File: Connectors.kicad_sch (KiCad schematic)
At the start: 4 parts

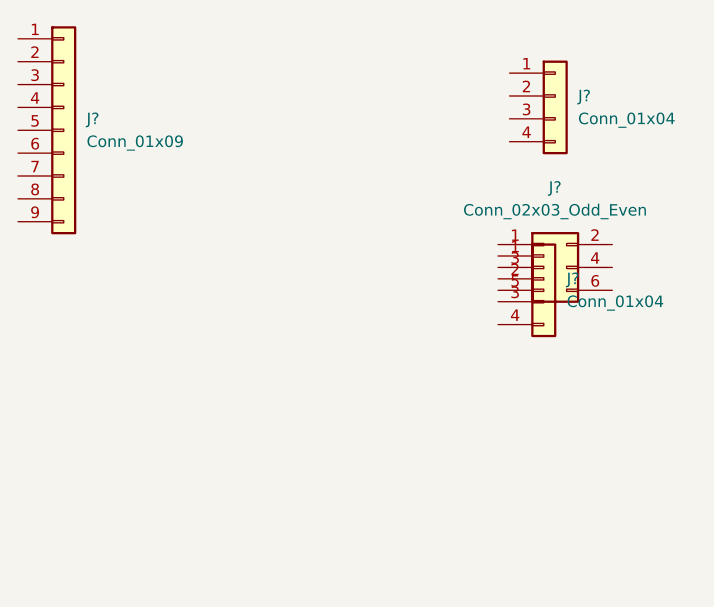
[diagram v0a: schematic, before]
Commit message: Annotation
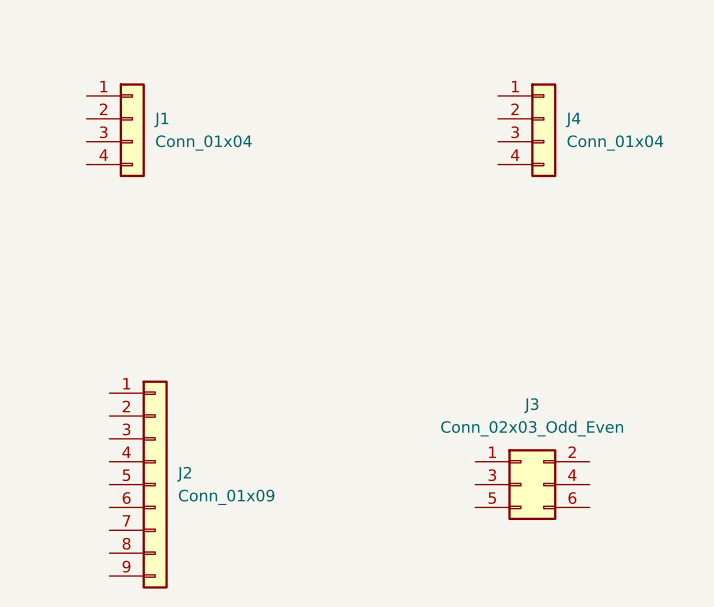
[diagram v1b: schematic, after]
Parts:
- gave numbers to parts that had none: 4
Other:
- moved on the sheet: J1, J2, J3, J4
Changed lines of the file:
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@@
     (company "GM Industries")
   )
-  (symbol (lib_id "Connector_Generic:Conn_01x09") (at 91.44 59.69 0) (unit 1)
+  (symbol (lib_id "Connector_Generic:Conn_01x09") (at 101.6 99.06 0) (unit 1)
     (in_bom yes) (on_board yes) (fields_autoplaced)
-    (property "Reference" "J?" (id 0) (at 93.98 58.4199 0)
+    (property "Reference" "J2" (id 0) (at 104.14 97.7899 0)
       (effects (font (size 1.27 1.27)) (justify left))
     )
-    (property "Value" "Conn_01x09" (id 1) (at 93.98 60.9599 0)
+    (property "Value" "Conn_01x09" (id 1) (at 104.14 100.3299 0)
       (effects (font (size 1.27 1.27)) (justify left))
     )
-    (property "Footprint" "" (id 2) (at 91.44 59.69 0)
+    (property "Footprint" "" (id 2) (at 101.6 99.06 0)
       (effects (font (size 1.27 1.27)) hide)
     )
-    (property "Datasheet" "~" (id 3) (at 91.44 59.69 0)
+    (property "Datasheet" "~" (id 3) (at 101.6 99.06 0)
       (effects (font (size 1.27 1.27)) hide)
     )
@@
     (pin "9")
   )
-  (symbol (lib_id "Connector_Generic:Conn_02x03_Odd_Even") (at 144.78 74.93 0) (unit 1)
+  (symbol (lib_id "Connector_Generic:Conn_02x03_Odd_Even") (at 142.24 99.06 0) (unit 1)
     (in_bom yes) (on_board yes) (fields_autoplaced)
-    (property "Reference" "J?" (id 0) (at 146.05 66.04 0))
-    (property "Value" "Conn_02x03_Odd_Even" (id 1) (at 146.05 68.58 0))
-    (property "Footprint" "" (id 2) (at 144.78 74.93 0)
+    (property "Reference" "J3" (id 0) (at 143.51 90.17 0))
+    (property "Value" "Conn_02x03_Odd_Even" (id 1) (at 143.51 92.71 0))
+    (property "Footprint" "" (id 2) (at 142.24 99.06 0)
       (effects (font (size 1.27 1.27)) hide)
     )
-    (property "Datasheet" "~" (id 3) (at 144.78 74.93 0)
+    (property "Datasheet" "~" (id 3) (at 142.24 99.06 0)
       (effects (font (size 1.27 1.27)) hide)
     )
@@
     (pin "6")
   )
-  (symbol (lib_id "Connector_Generic:Conn_01x04") (at 144.78 76.2 0) (unit 1)
+  (symbol (lib_id "Connector_Generic:Conn_01x04") (at 144.78 58.42 0) (unit 1)
     (in_bom yes) (on_board yes) (fields_autoplaced)
-    (property "Reference" "J?" (id 0) (at 147.32 76.1999 0)
+    (property "Reference" "J4" (id 0) (at 147.32 58.4199 0)
       (effects (font (size 1.27 1.27)) (justify left))
     )
-    (property "Value" "Conn_01x04" (id 1) (at 147.32 78.7399 0)
+    (property "Value" "Conn_01x04" (id 1) (at 147.32 60.9599 0)
       (effects (font (size 1.27 1.27)) (justify left))
     )
-    (property "Footprint" "" (id 2) (at 144.78 76.2 0)
+    (property "Footprint" "" (id 2) (at 144.78 58.42 0)
       (effects (font (size 1.27 1.27)) hide)
     )
-    (property "Datasheet" "~" (id 3) (at 144.78 76.2 0)
+    (property "Datasheet" "~" (id 3) (at 144.78 58.42 0)
       (effects (font (size 1.27 1.27)) hide)
     )
@@
     (pin "4")
   )
-  (symbol (lib_id "Connector_Generic:Conn_01x04") (at 146.05 55.88 0) (unit 1)
+  (symbol (lib_id "Connector_Generic:Conn_01x04") (at 99.06 58.42 0) (unit 1)
     (in_bom yes) (on_board yes) (fields_autoplaced)
-    (property "Reference" "J?" (id 0) (at 148.59 55.8799 0)
+    (property "Reference" "J1" (id 0) (at 101.6 58.4199 0)
       (effects (font (size 1.27 1.27)) (justify left))
     )
-    (property "Value" "Conn_01x04" (id 1) (at 148.59 58.4199 0)
+    (property "Value" "Conn_01x04" (id 1) (at 101.6 60.9599 0)
       (effects (font (size 1.27 1.27)) (justify left))
     )
-    (property "Footprint" "" (id 2) (at 146.05 55.88 0)
+    (property "Footprint" "" (id 2) (at 99.06 58.42 0)
       (effects (font (size 1.27 1.27)) hide)
     )
-    (property "Datasheet" "~" (id 3) (at 146.05 55.88 0)
+    (property "Datasheet" "~" (id 3) (at 99.06 58.42 0)
       (effects (font (size 1.27 1.27)) hide)
     )
